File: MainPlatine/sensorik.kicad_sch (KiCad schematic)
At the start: 10 parts, among them J1 Conn_01x07_Pin, J4 Conn_01x03_Pin

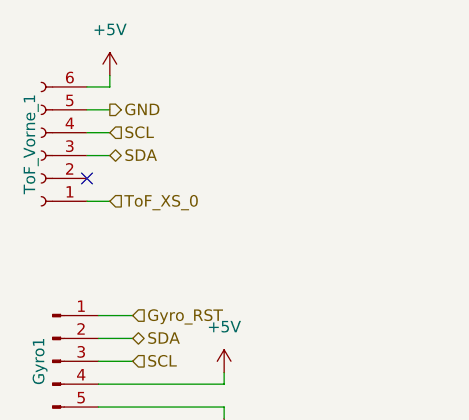
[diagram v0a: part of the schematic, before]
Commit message: fix main pcb
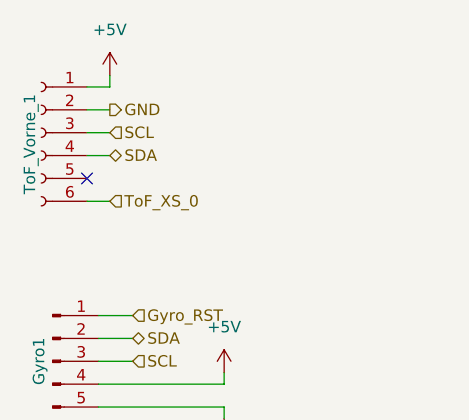
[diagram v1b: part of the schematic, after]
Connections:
- net +5V: now also ToF_Vorne_1.1 (Pin_1); no longer ToF_Vorne_1.6 (Pin_6)
- net GND: now also ToF_Vorne_1.2 (Pin_2); no longer ToF_Vorne_1.5 (Pin_5)
- net SCL: now also ToF_Vorne_1.3 (Pin_3); no longer ToF_Vorne_1.4 (Pin_4)
- net SDA: now also ToF_Vorne_1.4 (Pin_4); no longer ToF_Vorne_1.3 (Pin_3)
- net ToF_XS_0: now also ToF_Vorne_1.6 (Pin_6); no longer ToF_Vorne_1.1 (Pin_1)
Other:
- moved on the sheet: ToF_Vorne_1
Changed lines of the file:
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@@
 	(symbol
 		(lib_id "Connector:Conn_01x06_Socket")
-		(at 68.58 69.85 180)
+		(at 68.58 67.31 0)
+		(mirror y)
 		(unit 1)
 		(exclude_from_sim no)
@@
 		)
 		(property "Value" "Conn_01x06_Socket"
-			(at 69.215 59.69 0)
+			(at 69.215 77.47 0)
 			(effects
 				(font
@@
 		)
 		(property "Footprint" "Connector_PinSocket_2.54mm:PinSocket_1x06_P2.54mm_Horizontal"
-			(at 68.58 69.85 0)
+			(at 68.58 67.31 0)
 			(effects
 				(font
@@
 		)
 		(property "Datasheet" "~"
-			(at 68.58 69.85 0)
+			(at 68.58 67.31 0)
 			(effects
 				(font
@@
 		)
 		(property "Description" "Generic connector, single row, 01x06, script generated"
-			(at 68.58 69.85 0)
+			(at 68.58 67.31 0)
 			(effects
 				(font

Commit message: update new
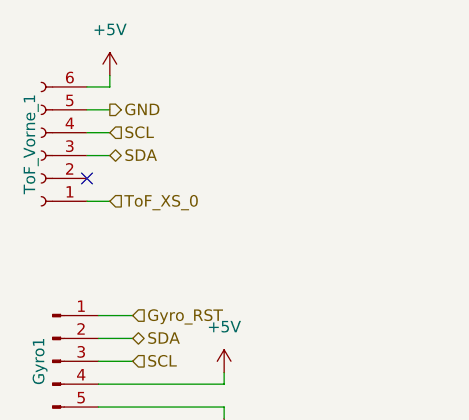
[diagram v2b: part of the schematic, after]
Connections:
- net +5V: now also ToF_Vorne_1.6 (Pin_6); no longer ToF_Vorne_1.1 (Pin_1)
- net GND: now also ToF_Vorne_1.5 (Pin_5); no longer ToF_Vorne_1.2 (Pin_2)
- net SCL: now also ToF_Vorne_1.4 (Pin_4); no longer ToF_Vorne_1.3 (Pin_3)
- net SDA: now also ToF_Vorne_1.3 (Pin_3); no longer ToF_Vorne_1.4 (Pin_4)
- net ToF_XS_0: now also ToF_Vorne_1.1 (Pin_1); no longer ToF_Vorne_1.6 (Pin_6)
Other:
- moved on the sheet: ToF_Vorne_1
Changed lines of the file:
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@@
 	(symbol
 		(lib_id "Connector:Conn_01x06_Socket")
-		(at 68.58 67.31 0)
-		(mirror y)
+		(at 68.58 69.85 180)
 		(unit 1)
 		(exclude_from_sim no)
@@
 		)
 		(property "Value" "Conn_01x06_Socket"
-			(at 69.215 77.47 0)
+			(at 69.215 59.69 0)
 			(effects
 				(font
@@
 		)
 		(property "Footprint" "Connector_PinSocket_2.54mm:PinSocket_1x06_P2.54mm_Horizontal"
-			(at 68.58 67.31 0)
+			(at 68.58 69.85 0)
 			(effects
 				(font
@@
 		)
 		(property "Datasheet" "~"
-			(at 68.58 67.31 0)
+			(at 68.58 69.85 0)
 			(effects
 				(font
@@
 		)
 		(property "Description" "Generic connector, single row, 01x06, script generated"
-			(at 68.58 67.31 0)
+			(at 68.58 69.85 0)
 			(effects
 				(font
